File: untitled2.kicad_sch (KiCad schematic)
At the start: 108 parts, among them U10 TCRT5000L, U11 TCRT5000L, U28 QRE1113GR, U29 QRE1113GR, U3 TCRT5000L, U30 QRE1113GR, U31 QRE1113GR, U32 QRE1113GR, U33 QRE1113GR, U34 QRE1113GR, U35 QRE1113GR, U36 QRE1113GR, U4 TCRT5000L, U5 TCRT5000L, U6 TCRT5000L, U7 TCRT5000L, U8 TCRT5000L, U9 TCRT5000L

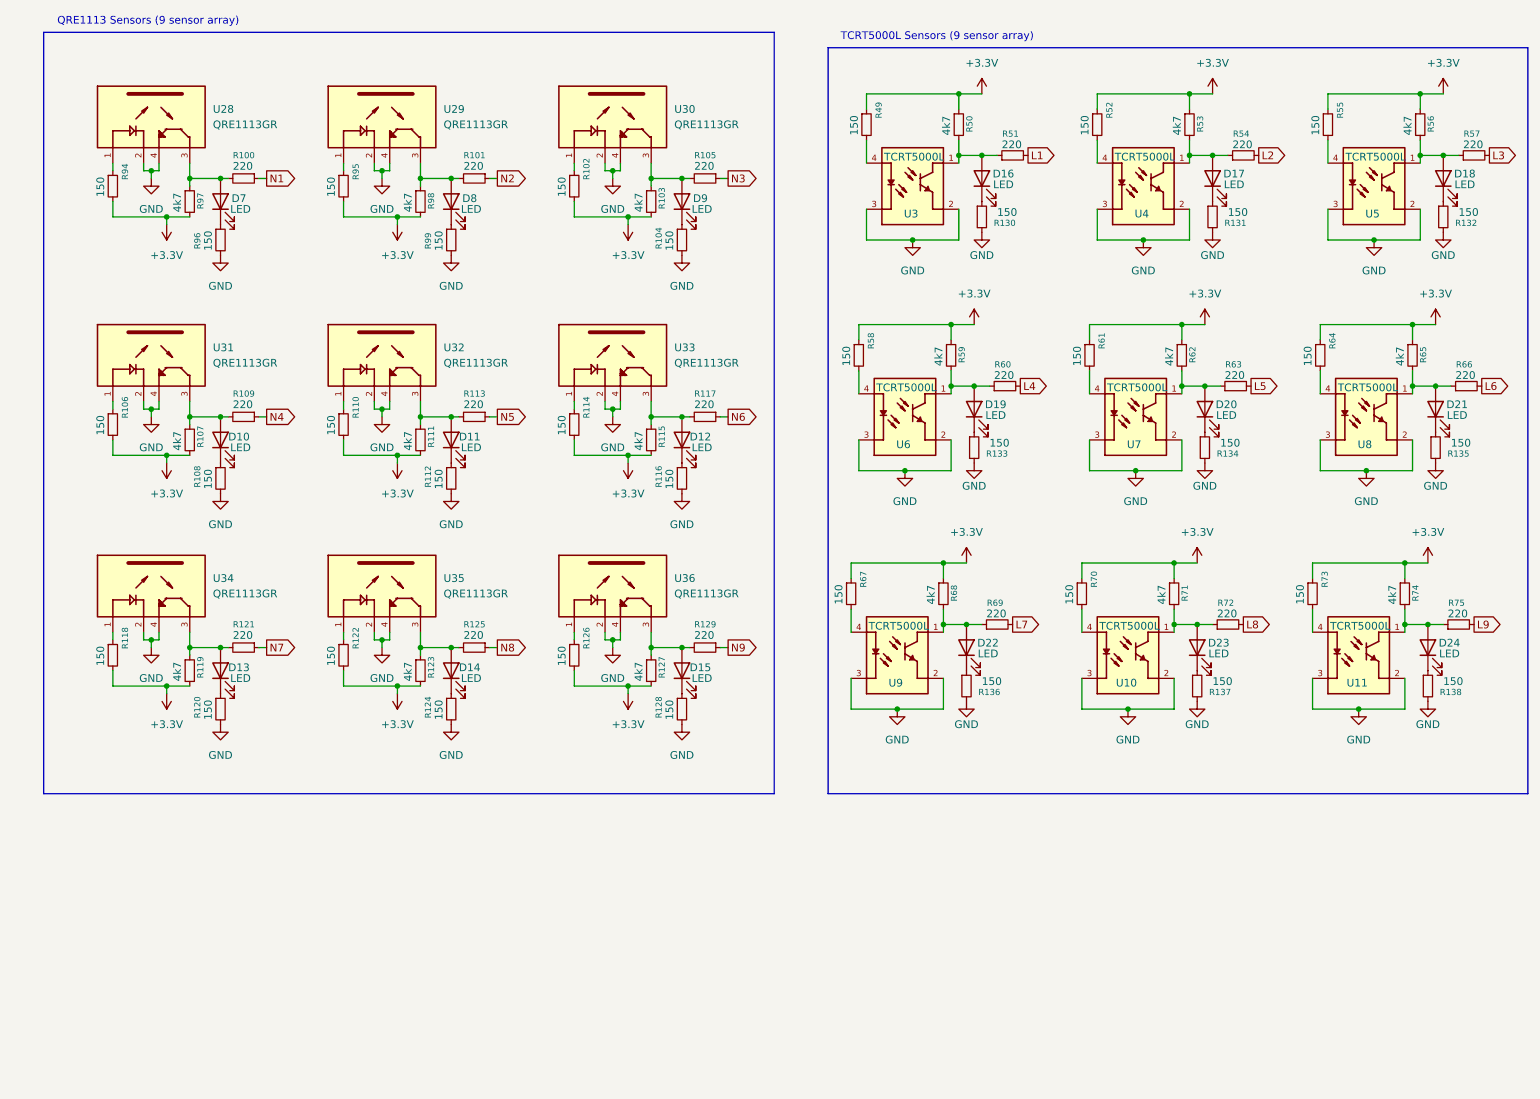
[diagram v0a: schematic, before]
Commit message: PCB
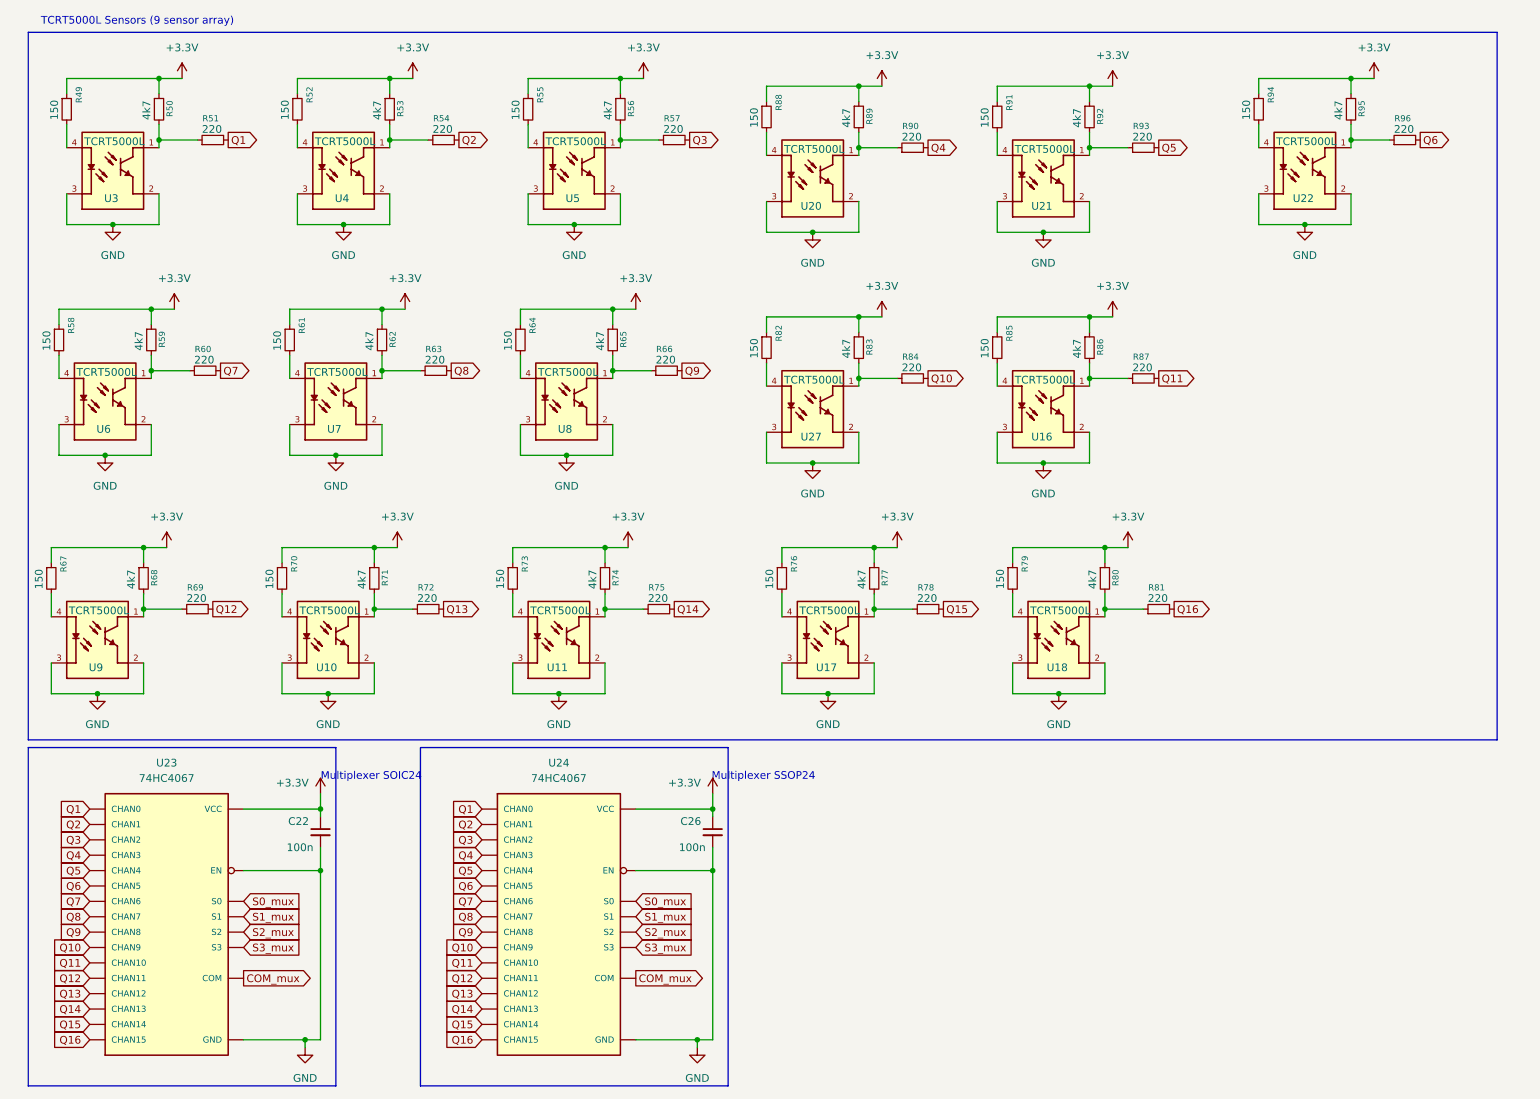
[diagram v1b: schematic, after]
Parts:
- removed D10, D11, D12, D13, D14, D15, D16, D17, D18, D19, D20, D21, D22, D23, D24, D7, D8, D9: LED, LED_THT:LED_D3.0mm, symbol Device:LED
- removed R100, R101, R105, R109, R113, R117, R121, R125, R129: 220, Resistor_SMD:R_0603_1608Metric_Pad0.98x0.95mm_HandSolder, symbol Device:R_Small
- removed R102, R104, R106, R108, R110, R112, R114, R116, R118, R120, R122, R124, R126, R128, R130, R131, R132, R133, R134, R135, R136, R137, R138, R99: 150, Resistor_SMD:R_0603_1608Metric_Pad0.98x0.95mm_HandSolder, symbol Device:R_Small
- removed R103, R107, R111, R115, R119, R123, R127, R97, R98: 4k7, Resistor_SMD:R_0603_1608Metric_Pad0.98x0.95mm_HandSolder, symbol Device:R_Small
- removed U28, U29, U30, U31, U32, U33, U34, U35, U36: QRE1113GR, MyCustoms:QRE1113-SMD, symbol customs:QRE1113GR
- added C22, C26: 100n, Capacitor_SMD:C_0603_1608Metric_Pad1.08x0.95mm_HandSolder, symbol Device:C_Small
- added R76, R79, R82, R85, R88, R91: 150, Resistor_SMD:R_0603_1608Metric_Pad0.98x0.95mm_HandSolder, symbol Device:R_Small
- added R77, R80, R83, R86, R89, R92: 4k7, Resistor_SMD:R_0603_1608Metric_Pad0.98x0.95mm_HandSolder, symbol Device:R_Small
- added R78, R81, R84, R87, R90, R93: 220, Resistor_SMD:R_0603_1608Metric_Pad0.98x0.95mm_HandSolder, symbol Device:R_Small
- added U16, U17, U18, U20, U21, U22, U27: TCRT5000L, CustomLibrary:XDCR_TCRT5000L, symbol customs:TCRT5000L
- added U23: 74HC4067, Package_SO:SOIC-24W_7.5x15.4mm_P1.27mm, symbol customs:74HC4067
- added U24: 74HC4067, Package_SO:TSSOP-24_4.4x7.8mm_P0.65mm, symbol customs:74HC4067
- R95: value 150 -> 4k7
- R96: value 150 -> 220
- U10, U11, U3, U4, U5, U6, U7, U8, U9: footprint MyCustoms:XDCR_TCRT5000L -> CustomLibrary:XDCR_TCRT5000L
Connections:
- net +3.3V: now also R94.1, R95.1, C22.1, C26.1, R76.1, R77.1, R79.1, R80.1, R82.1, R83.1, R85.1, R86.1, R88.1, R89.1, R91.1, R92.1, U23.24 (VCC), U24.24 (VCC); no longer R94.2, R95.2
- net GND: now also C22.2, C26.2, U16.2, U16.3, U17.2, U17.3, U18.2, U18.3, U20.2, U20.3, U21.2, U21.3, U22.2, U22.3, U23.12 (GND), U23.15 (EN), U24.12 (GND), U24.15 (EN), U27.2, U27.3; no longer R96.2
- net at R96.1: now also R95.2, U22.1
- net L1 renamed Q1
- net Q1: now also U23.9 (CHAN0), U24.9 (CHAN0)
- net L2 renamed Q2
- net Q2: now also U23.8 (CHAN1), U24.8 (CHAN1)
- net L3 renamed Q3
- net Q3: now also U23.7 (CHAN2), U24.7 (CHAN2)
- net L4 renamed Q7
- net Q7: now also U23.3 (CHAN6), U24.3 (CHAN6)
- net L5 renamed Q8
- net Q8: now also U23.2 (CHAN7), U24.2 (CHAN7)
- net L6 renamed Q9
- net Q9: now also U23.23 (CHAN8), U24.23 (CHAN8)
- net L7 renamed Q12
- net Q12: now also U23.20 (CHAN11), U24.20 (CHAN11)
- net L8 renamed Q13
- net Q13: now also U23.19 (CHAN12), U24.19 (CHAN12)
- net L9 renamed Q14
- net Q14: now also U23.18 (CHAN13), U24.18 (CHAN13)
- new net: R83.2, R84.1, U27.1
- new net: R82.2, U27.4
- new net: R91.2, U21.4
- new net: R92.2, R93.1, U21.1
- new net: R80.2, R81.1, U18.1
- new net: R88.2, U20.4
- new net: R85.2, U16.4
- new net: R94.2, U22.4
- new net: R86.2, R87.1, U16.1
- new net: R76.2, U17.4
- new net: R79.2, U18.4
- new net: R89.2, R90.1, U20.1
- new net: R77.2, R78.1, U17.1
- new net COM_mux: U23.1 (COM), U24.1 (COM)
- new net Q10: R84.2, U23.22 (CHAN9), U24.22 (CHAN9)
- new net Q11: R87.2, U23.21 (CHAN10), U24.21 (CHAN10)
- new net Q15: R78.2, U23.17 (CHAN14), U24.17 (CHAN14)
- new net Q16: R81.2, U23.16 (CHAN15), U24.16 (CHAN15)
- new net Q4: R90.2, U23.6 (CHAN3), U24.6 (CHAN3)
- new net Q5: R93.2, U23.5 (CHAN4), U24.5 (CHAN4)
- new net Q6: R96.2, U23.4 (CHAN5), U24.4 (CHAN5)
- new net S0_mux: U23.10 (S0), U24.10 (S0)
- new net S1_mux: U23.11 (S1), U24.11 (S1)
- new net S2_mux: U23.14 (S2), U24.14 (S2)
- new net S3_mux: U23.13 (S3), U24.13 (S3)
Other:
- note added: "Multiplexer SOIC24"
- note added: "Multiplexer SSOP24"
- note removed: "QRE1113 Sensors (9 sensor array)"
- moved on the sheet: R49, R50, R51, R52, R53, R54, R55, R56, R57, R58, R59, R60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
